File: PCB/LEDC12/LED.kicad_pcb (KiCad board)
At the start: 2 copper layers, 70 x 70 mm, 38 parts, among them J1 Reset, J2 Wago, J3 USB-C-Socket-H, J4 TC2030-USB-NL-DS, SW1 Button, U1 ESP32-S3-MINI-1, U2 IRMHF384, U3 ICS43434_MEMS_Mic, U4 TPS562243

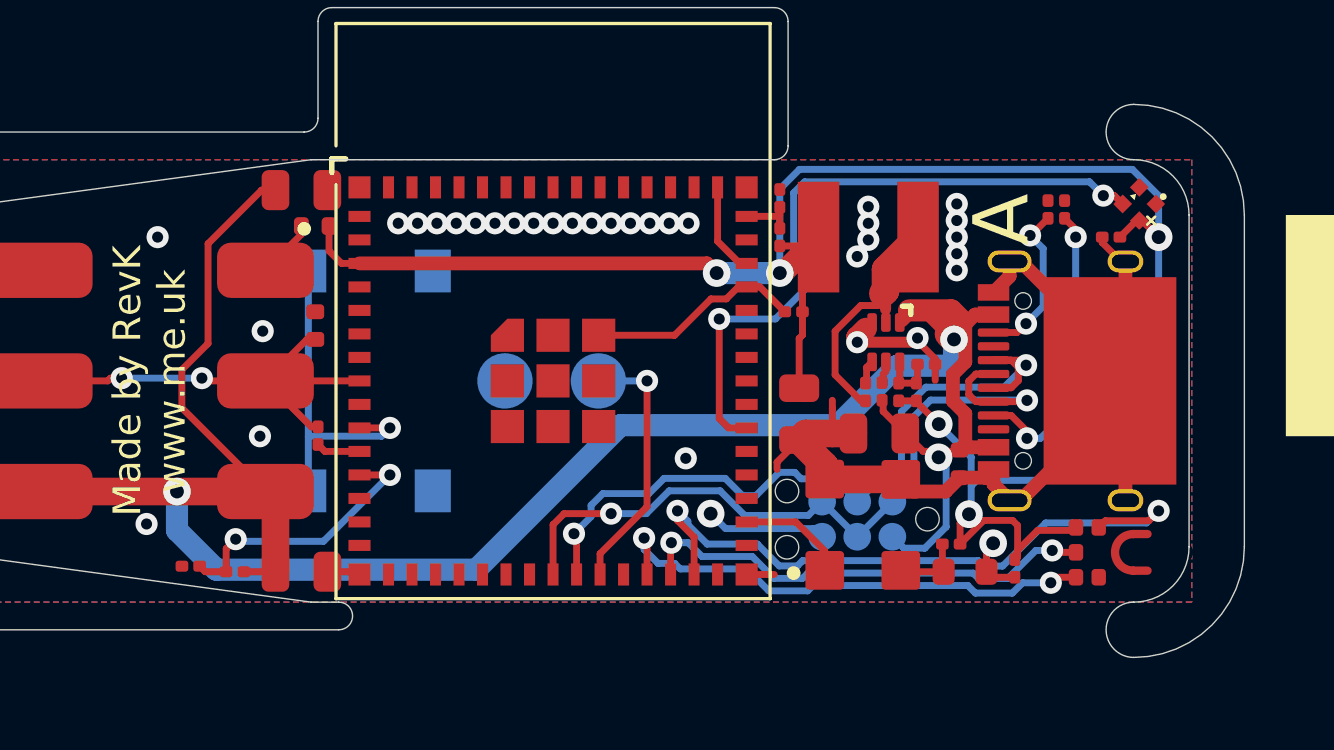
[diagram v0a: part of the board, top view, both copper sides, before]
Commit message: Margins tidy
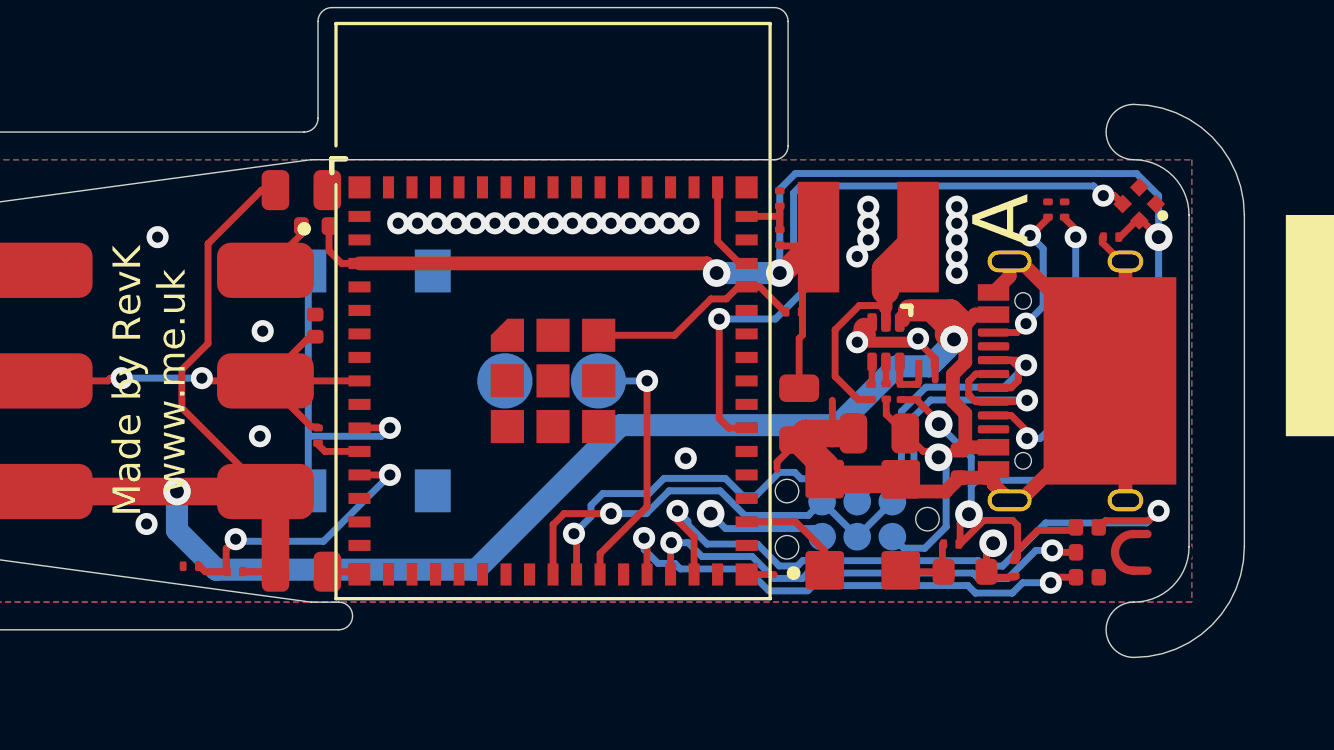
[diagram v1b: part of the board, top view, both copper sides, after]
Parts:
- R8: value 100k -> 150k 1%
- moved C12 0.20 mm to (110.0, 100.4)
- moved R8 0.15 mm to (110.5, 100.4), turned to -90 degrees
- moved R9 0.10 mm to (111.1, 100.4)
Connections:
- R8 pad 1: DC -> EN
- R8 pad 2: EN -> DC
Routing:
- net SW: track 9.43 -> 11.0 mm
